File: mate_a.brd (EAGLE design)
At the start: 92.7 x 100 mm, 8 parts, among them IC1 PIC18F47Q84-E_P, X1 GLX-S-88M

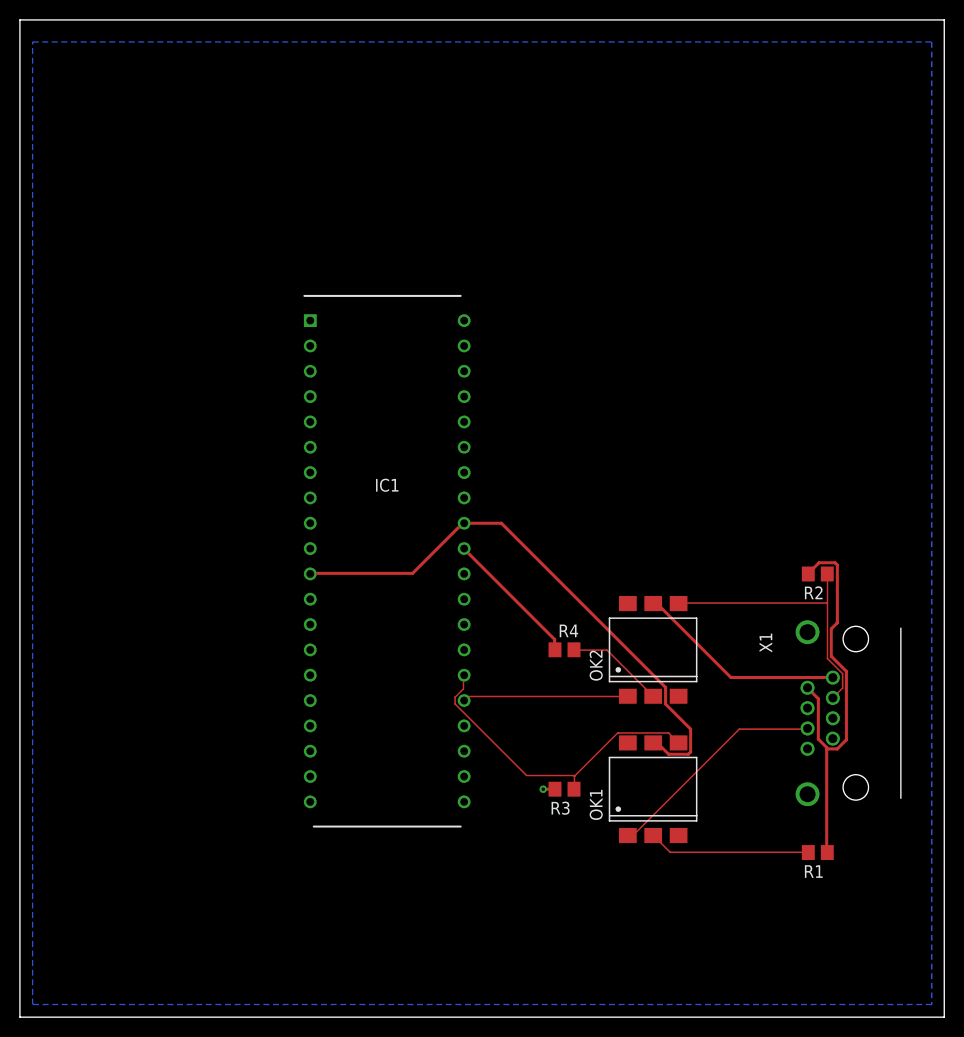
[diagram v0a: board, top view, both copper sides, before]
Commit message: up
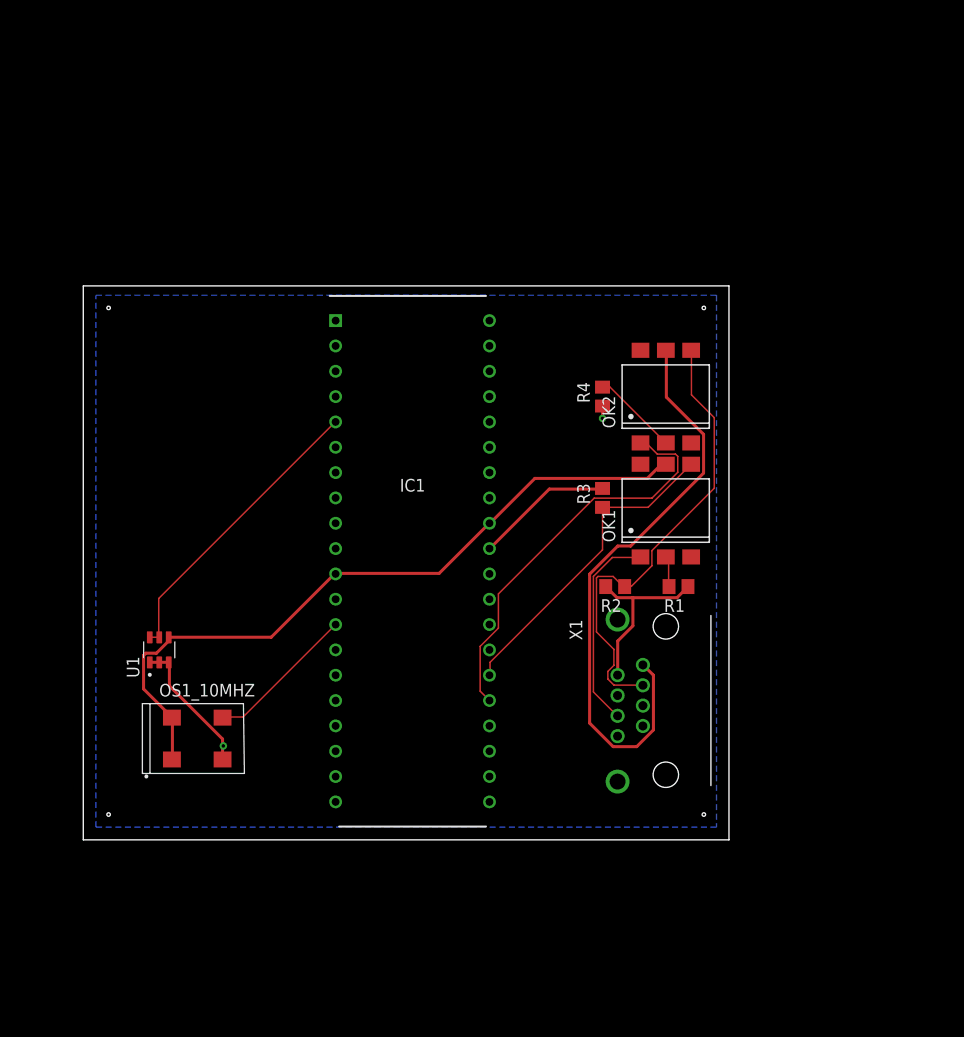
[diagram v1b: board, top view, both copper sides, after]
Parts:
- added OS1_10MHZ: OSC-OE-CFPS-72, IQD-Frequency-Products:7.2X5.2-4-PAD
- added U1: REF3440IDBVR, REF3440IDBVR:SOT95P280X145-6N
- moved R1 30.1 mm to (133.3, 43.2)
- moved R3 29.5 mm to (125.7, 52.1), turned to 90 degrees
- moved OK1 28.0 mm to (132.1, 50.8)
- moved R4 25.7 mm to (125.7, 62.2), turned to 90 degrees
- moved OK2 25.4 mm to (132.1, 62.2)
- moved R2 20.4 mm to (127.0, 43.2)
- moved X1 19.1 mm to (132.1, 31.8)
- moved IC1 2.54 mm to (106.7, 45.7)
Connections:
- new net CPU_CLK: IC1.13, OS1_10MHZ.3
- new net VREF: IC1.5, U1.5, U1.6
- net VDD: now also OS1_10MHZ.1, OS1_10MHZ.4, U1.4
- net VSS: now also OS1_10MHZ.2, U1.1, U1.2, U1.3
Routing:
- net +24V: track 21.1 -> 59.5 mm
- net VREF: track 0.00 -> 29.9 mm
- net PC_TX: track 16.6 -> 40.8 mm
- net 0V: track 41.6 -> 17.6 mm
- net MX_TX: track 28.5 -> 47.0 mm
- net VDD: track 56.4 -> 72.2 mm
- net CPU_CLK: track 0.00 -> 15.2 mm
- net VSS: track 15.1 -> 29.0 mm, vias 1 -> 2
- net N$1: track 16.3 -> 3.11 mm
- net MX_RX: track 22.5 -> 20.6 mm
- net N$3: track 9.86 -> 8.67 mm
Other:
- board size 92.7 x 100 mm -> 64.8 x 55.5 mm
